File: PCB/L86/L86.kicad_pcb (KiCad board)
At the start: 2 copper layers, 38.5 x 30 mm, 4 parts, among them J1 Conn_01x06, U1 L86-M33, U2 QR

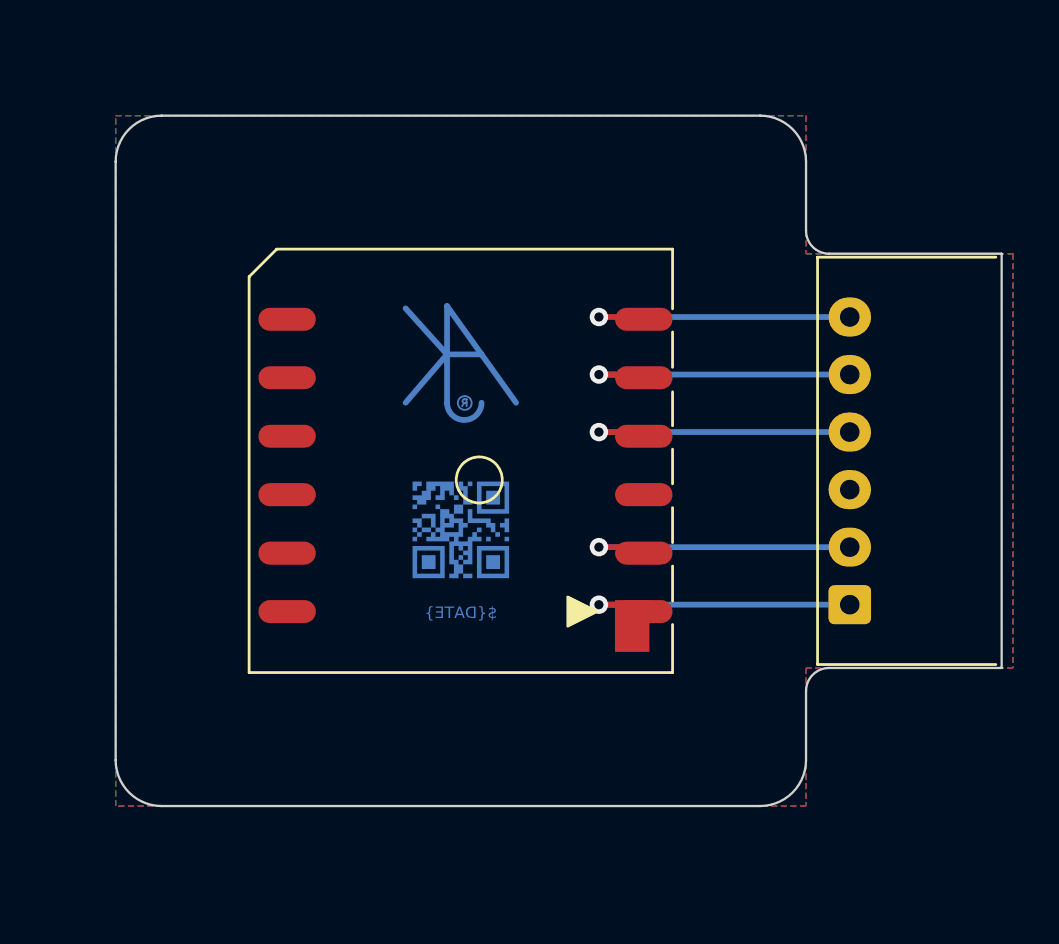
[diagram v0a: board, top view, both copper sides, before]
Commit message: Moved from SS
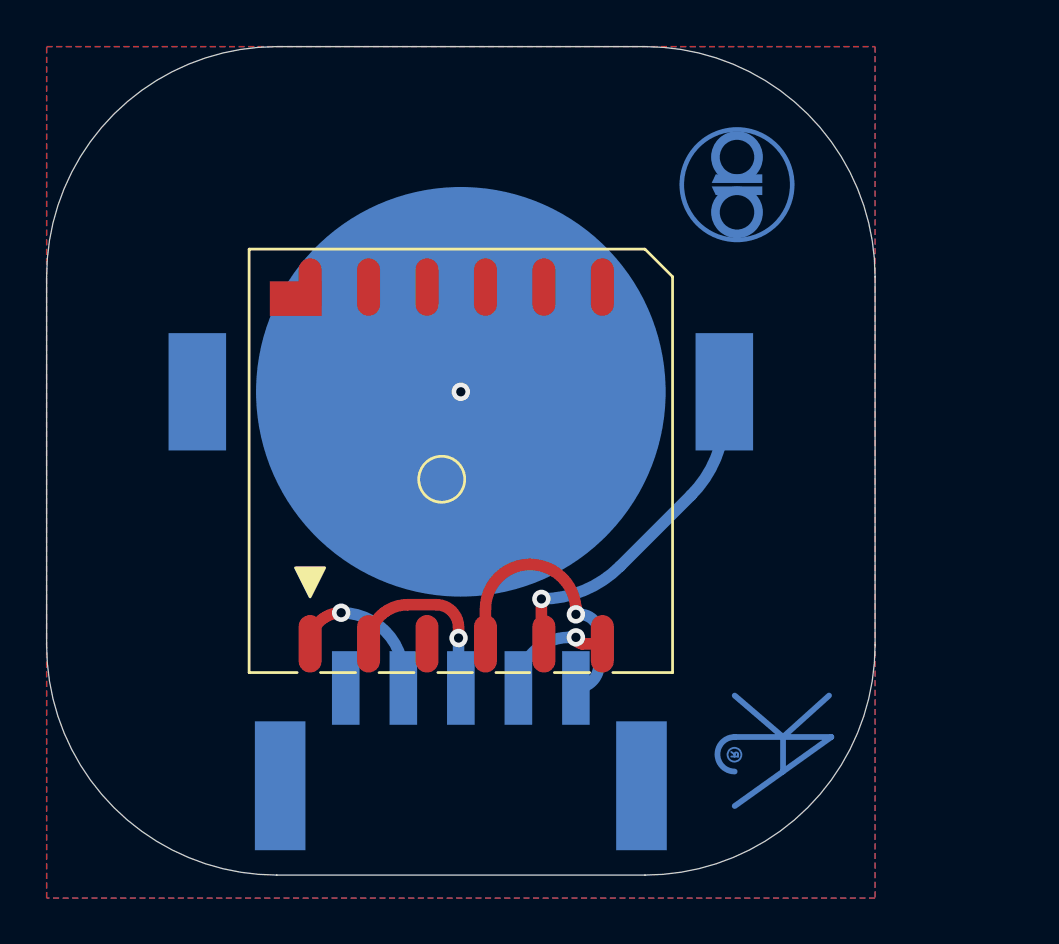
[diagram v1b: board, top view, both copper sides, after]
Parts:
- removed U2: QR, RevK:QR-GPS
- added BT1: Battery_Cell, RevK:Battery-Holder-2032, B.Cu at (100.0, 97.0)
- added Logo2: AJK, RevK:AJK, B.Cu at (114.0, 112.0)
- J1: value Conn_01x06 -> Conn_01x05; footprint RevK:Molex_MiniSPOX_H6RA -> RevK:PTSM-HH-5-RA-P-SMD; moved to B.Cu
- Logo1: value AJK -> AA; footprint RevK:AJK -> RevK:AA
- moved J1 19.6 mm to (100.0, 109.9), turned to 180 degrees
- moved Logo1 14.6 mm to (112.0, 88.0), turned to 90 degrees
- turned U1 to -90 degrees
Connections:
- J1 pad 1: Net-(J1-Pad1) -> GND
- J1 pad 2: Net-(J1-Pad2) -> Net-(J1-Pin_2)
- J1 pad 3: GND -> Net-(J1-Pin_3)
- J1 pad 4: Net-(J1-Pad4) -> Net-(J1-Pin_4)
- J1 pad 5: Net-(J1-Pad5) -> Net-(J1-Pin_5)
- U1 pad 1: Net-(J1-Pad1) -> Net-(J1-Pin_2)
- U1 pad 12: unconnected-(U1-Pad12) -> GND
- U1 pad 2: Net-(J1-Pad2) -> Net-(J1-Pin_3)
- U1 pad 4: Net-(J1-Pad4) -> Net-(J1-Pin_5)
- U1 pad 5: Net-(J1-Pad5) -> BAT
- U1 pad 6: Net-(J1-Pad6) -> Net-(J1-Pin_4)
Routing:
- net BAT: track 0.00 -> 15.0 mm, vias 0 -> 1
- net Net-(J1-Pad1): track 13.0 -> 0.00 mm, vias 1 -> 0
- net Net-(J1-Pad2): track 13.0 -> 0.00 mm, vias 1 -> 0
- net Net-(J1-Pad4): track 12.9 -> 0.00 mm, vias 1 -> 0
- net Net-(J1-Pad5): track 12.9 -> 0.00 mm, vias 1 -> 0
- net Net-(J1-Pad6): track 12.9 -> 0.00 mm, vias 1 -> 0
- net Net-(J1-Pin_5): track 0.00 -> 12.1 mm, vias 0 -> 1
- net Net-(J1-Pin_3): track 0.00 -> 8.03 mm, vias 0 -> 1
- net Net-(J1-Pin_2): track 0.00 -> 6.77 mm, vias 0 -> 1
- net Net-(J1-Pin_4): track 0.00 -> 4.97 mm, vias 0 -> 1
- net GND: vias 0 -> 1
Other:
- board size 38.5 x 30 mm -> 36 x 36 mm
- rule pad_to_mask_clearance: 0.01 -> 0
- board text added: "${CURRENT_DATE}"
- board text added: "+"
- board text added: "<"
- board text added: ">"
- board text added: "GPS"
- board text added: "⎍"
- board text added: "⏚"
- board text removed: "BAT"
- board text removed: "GND"
- board text removed: "PPS"
- board text removed: "VCC"
- board text removed: "←TX"
- board text removed: "→RX"
